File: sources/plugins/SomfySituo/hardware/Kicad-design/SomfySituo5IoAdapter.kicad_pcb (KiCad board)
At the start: 2 copper layers, 68.6 x 66 mm, 30 parts, among them J1 USB_OTG, J10 Conn_01x01, J11 Conn_01x01, J12 Conn_01x01, J13 Conn_01x01, J2 Conn_01x01, J3 Conn_01x01, J4 Conn_01x01, J5 Conn_01x01, J6 Conn_01x01, J7 Conn_01x01, J8 Conn_01x01, J9 Conn_01x01, P1 ICSP_PicKit2, U1 FT230X, U2 PIC16F688

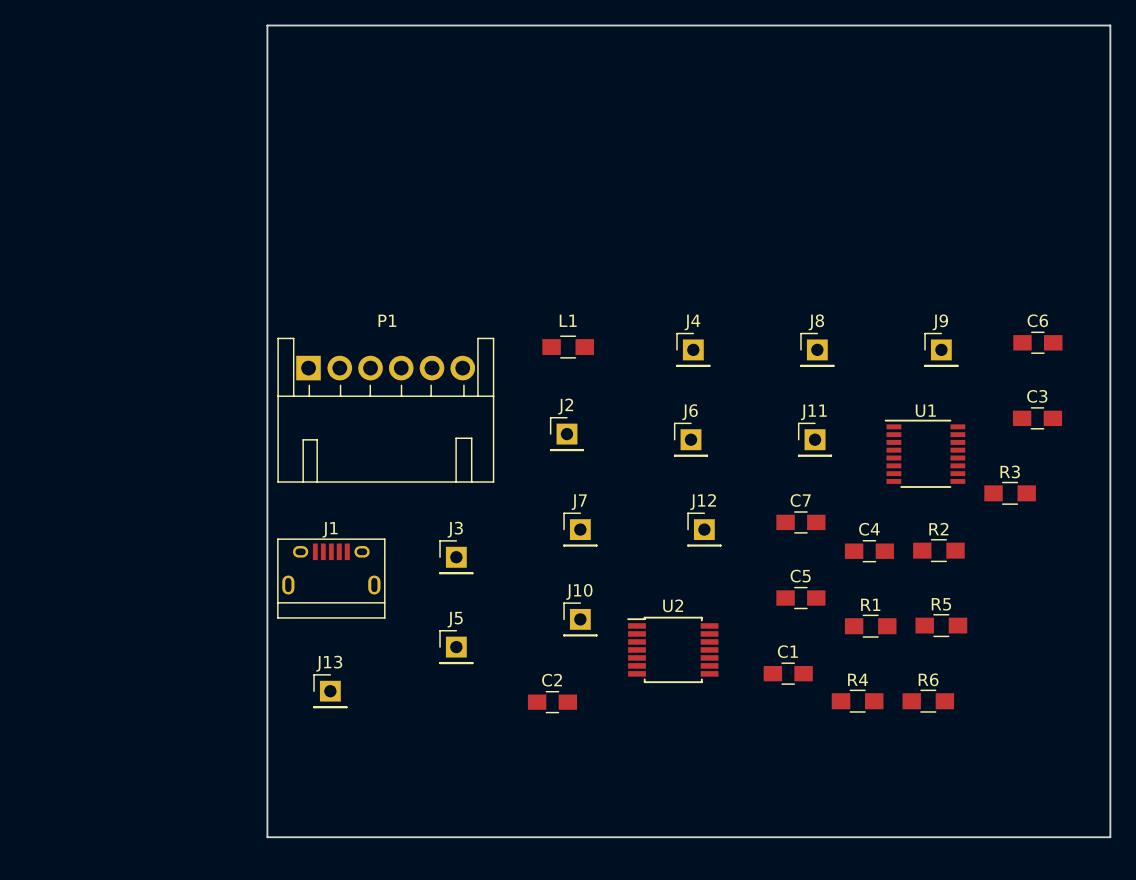
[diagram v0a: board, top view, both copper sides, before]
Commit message: Place components
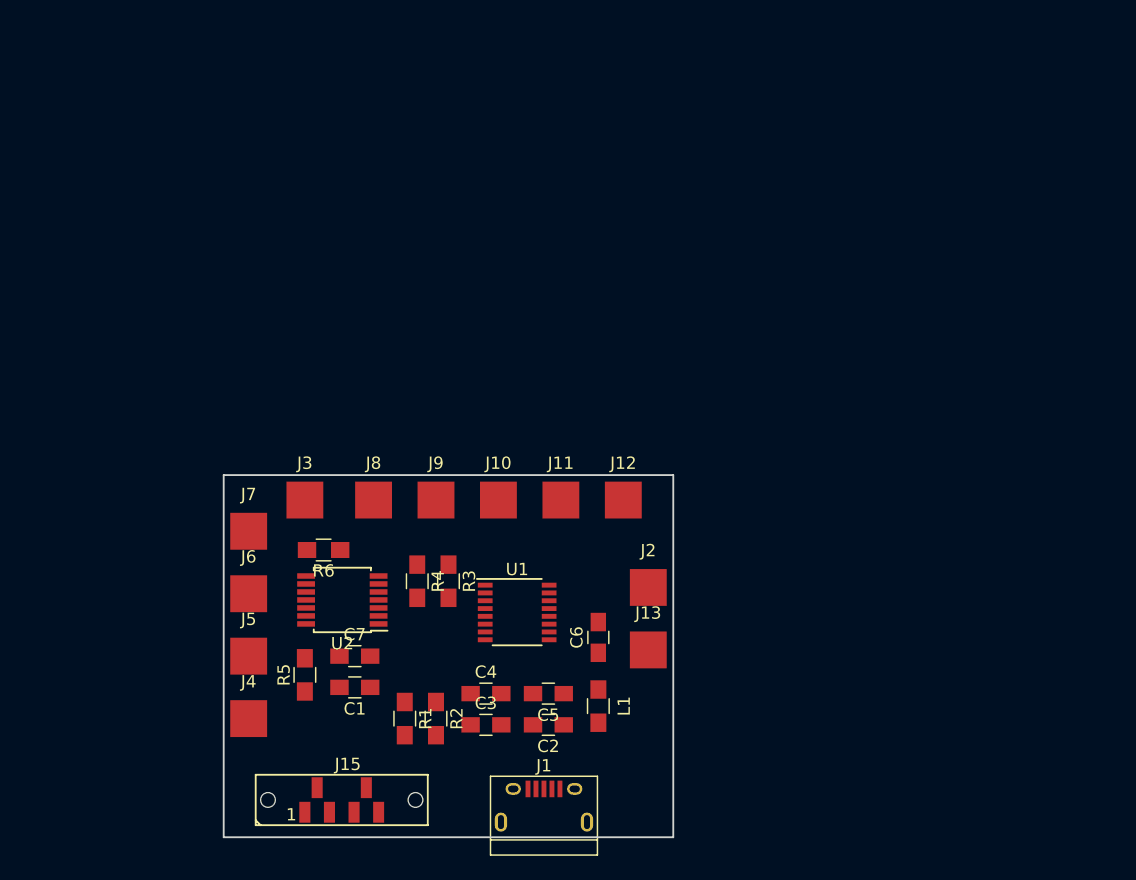
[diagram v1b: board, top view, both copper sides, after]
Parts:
- removed P1: ICSP_PicKit2, Connectors:Wafer_Horizontal17.5x5.8x7RM2.5-6
- added J15: ICSP, AVX 00-9188 006 receiver:AVX_00-9188_006_receiver, F.Cu at (130.0, 130.0)
- J10, J11, J12, J13, J2, J3, J4, J5, J6, J7, J8, J9: footprint Socket_Strips:Socket_Strip_Straight_1x01_Pitch2.54mm -> Measurement_Points:Measurement_Point_Square-SMD-Pad_Big
- moved R5 51.9 mm to (130.0, 118.9), turned to 90 degrees
- moved C3 51.3 mm to (144.8, 122.9)
- moved R6 50.7 mm to (131.6, 108.7), turned to 180 degrees
- moved J4 47.0 mm to (125.5, 122.4)
- moved R3 46.2 mm to (141.7, 111.3), turned to 270 degrees
- moved R2 43.1 mm to (140.7, 122.4), turned to 270 degrees
- moved C6 43.1 mm to (153.9, 115.8), turned to 90 degrees
- moved J9 42.9 mm to (140.7, 104.6)
- moved R1 38.6 mm to (138.2, 122.4), turned to 270 degrees
- moved J8 38.1 mm to (135.6, 104.6)
- moved J6 38.1 mm to (125.5, 112.3)
- moved C7 37.9 mm to (134.1, 117.3)
- moved R4 37.1 mm to (139.2, 111.3), turned to 270 degrees
- moved U1 35.7 mm to (147.3, 113.8)
- moved C1 35.3 mm to (134.1, 119.9), turned to 180 degrees
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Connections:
- U1 pad 14: Net-(U1-Pad14) -> (no net)
- U1 pad 15: Net-(U1-Pad15) -> (no net)
- U1 pad 16: Net-(U1-Pad16) -> (no net)
- U1 pad 7: Net-(U1-Pad7) -> (no net)
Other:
- board size 68.6 x 66 mm -> 36.6 x 29.5 mm

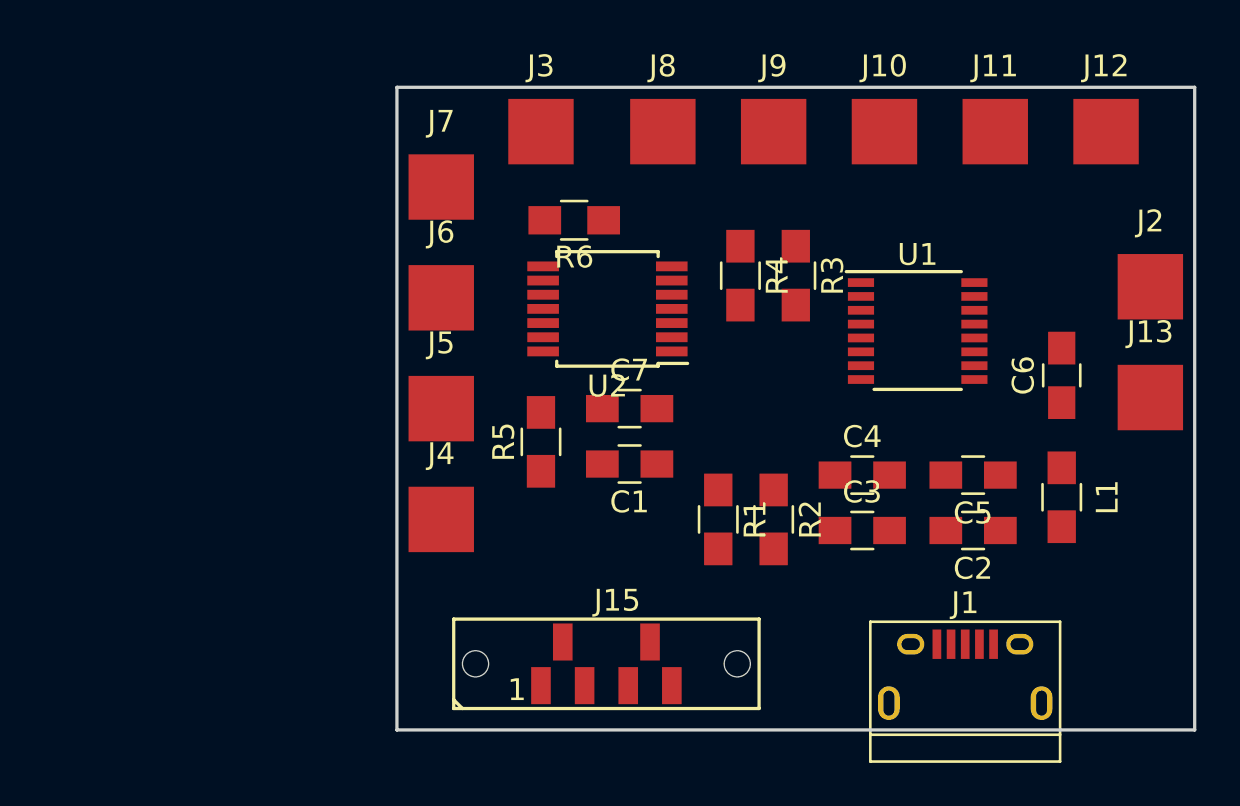
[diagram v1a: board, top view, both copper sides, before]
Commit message: Finish PCB
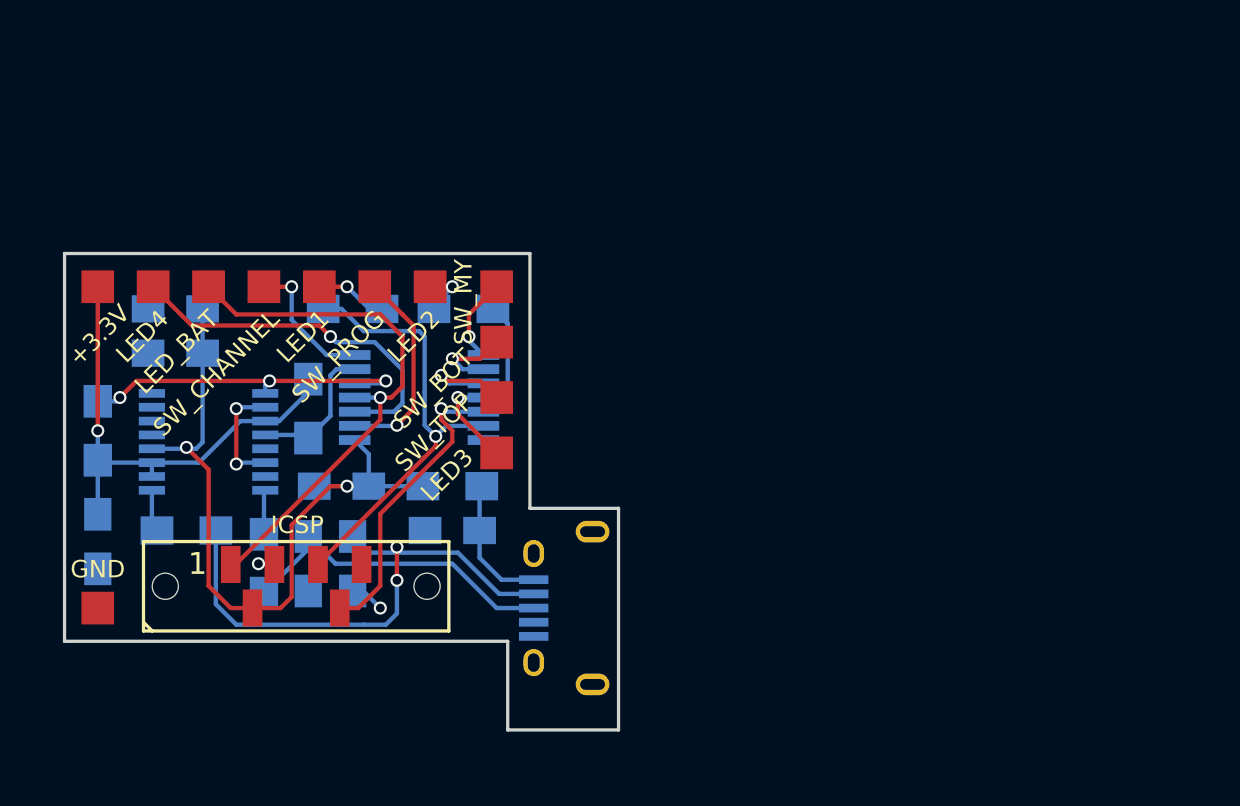
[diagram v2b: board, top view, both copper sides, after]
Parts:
- C1, C2, C3, C4, C5, C6, C7, J1, L1, R1, R2, R3, R4, R5, R6, U1, U2: moved to B.Cu
- J10, J11, J12, J13, J2, J3, J4, J5, J6, J7, J8, J9: footprint Measurement_Points:Measurement_Point_Square-SMD-Pad_Big -> Measurement_Points:Measurement_Point_Square-SMD-Pad_Small
- moved J13 49.2 mm to (109.7, 126.5)
- moved J2 48.3 mm to (109.7, 111.8)
- moved C6 40.8 mm to (113.3, 112.8), turned to 180 degrees
- moved C5 40.2 mm to (109.7, 123.4), turned to 270 degrees
- moved J11 34.3 mm to (117.3, 111.8)
- moved J12 34.3 mm to (122.4, 111.8)
- moved U1 32.9 mm to (114.8, 118.9), turned to 180 degrees
- moved R4 30.3 mm to (109.7, 118.4), turned to 90 degrees
- moved L1 27.9 mm to (126.0, 120.9), turned to 0 degrees
- moved R2 26.9 mm to (113.8, 122.9), turned to 0 degrees
- moved C3 25.4 mm to (119.4, 124.5), turned to 270 degrees
- moved C2 23.9 mm to (126.0, 122.9)
- moved C4 23.7 mm to (121.4, 124.5), turned to 270 degrees
- moved R3 23.2 mm to (119.4, 117.3)
- moved C1 21.4 mm to (113.3, 114.8)
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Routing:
- net VCC: track 0.00 -> 32.4 mm, vias 0 -> 2
- net ICSP_VPP: track 0.00 -> 25.1 mm, vias 0 -> 1
- net Net-(C4-Pad1): track 0.00 -> 25.0 mm, vias 0 -> 2
- net +3V3: track 0.00 -> 22.7 mm, vias 0 -> 1
- net ICSP_DATA: track 0.00 -> 20.7 mm, vias 0 -> 1
- net ICSP_CLK: track 0.00 -> 20.0 mm, vias 0 -> 1
- net Somfy_led4: track 0.00 -> 16.9 mm, vias 0 -> 1
- net Net-(R4-Pad2): track 0.00 -> 15.7 mm, vias 0 -> 3
- net Net-(C3-Pad1): track 0.00 -> 15.1 mm
- net Somfy_sw_prog: track 0.00 -> 9.35 mm, vias 0 -> 1
- net /VCC_IN: track 0.00 -> 6.91 mm
- net Net-(R3-Pad2): track 0.00 -> 6.56 mm
- net Somfy_sw_channel: track 0.00 -> 6.35 mm, vias 0 -> 1
- net Net-(U1-Pad2): track 0.00 -> 5.25 mm, vias 0 -> 2
- net Somfy_sw_top: track 0.00 -> 5.05 mm, vias 0 -> 1
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- added copper zone on B.Cu, net GND
- added copper zone on F.Cu, net GND
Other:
- board size 36.6 x 29.5 mm -> 25.4 x 21.8 mm
- net class Alim removed
- net class Default: trace_width 0.25 -> 0.2
- board text added: "+3.3V"
- board text added: "GND"
- board text added: "ICSP"
- board text added: "LED1"
- board text added: "LED2"
- board text added: "LED3"
- board text added: "LED4"
- board text added: "LED_BAT"
- board text added: "Recouper suivant taille réelle connecteur USB"
- board text added: "SW_BOT"
- board text added: "SW_CHANNEL"
- board text added: "SW_MY"
- board text added: "SW_PROG"
- board text added: "SW_TOP"
